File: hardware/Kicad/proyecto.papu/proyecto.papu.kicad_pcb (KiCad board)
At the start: 2 copper layers, 96.4 x 45.4 mm, 19 parts, among them J1 Conn_01x04, J2 Conn_01x03, J3 Screw_Terminal_01x02, J4 Screw_Terminal_01x02, J5 Screw_Terminal_01x02, SW1 SW_Nidec_CAS-120A1, SW2 SW_MEC_5E, U1 DRV8833_MODULE, U2 L7805

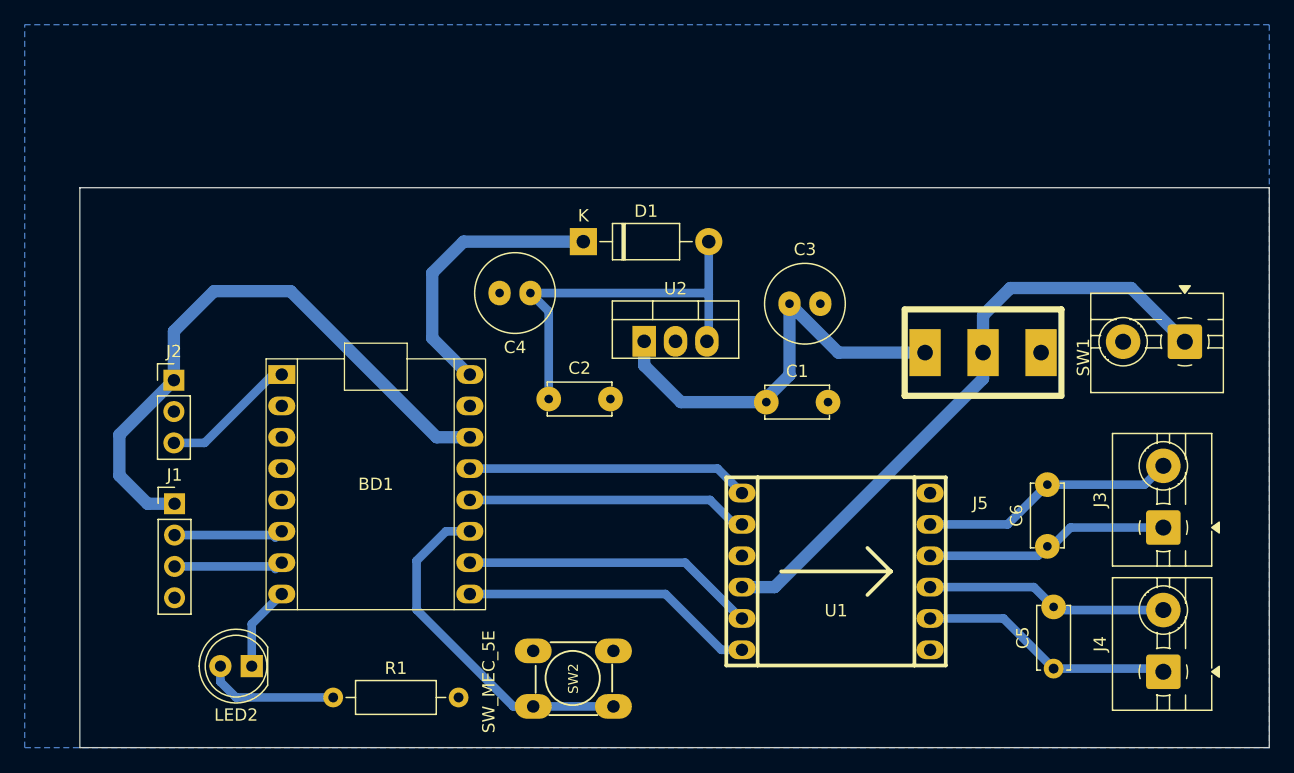
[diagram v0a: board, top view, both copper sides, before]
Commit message: se termino pcb
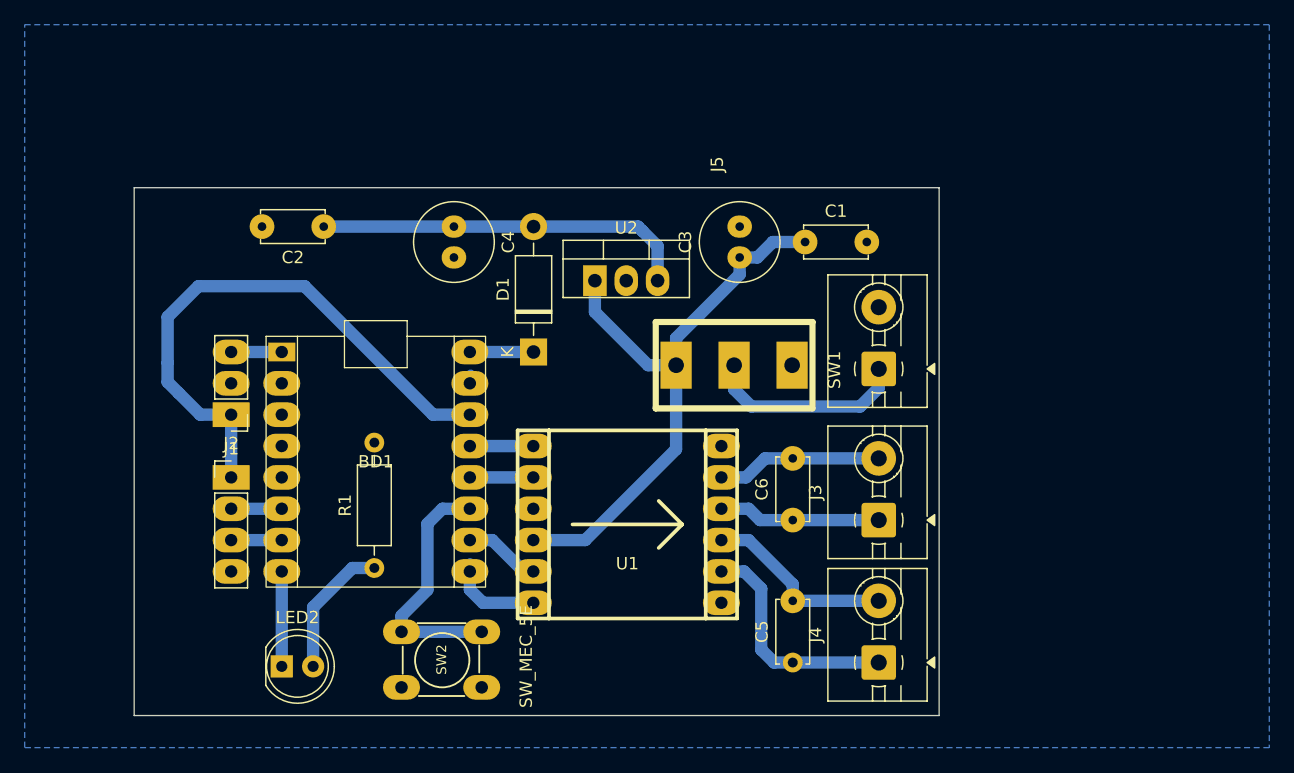
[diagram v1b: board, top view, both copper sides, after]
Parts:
- moved J5 24.9 mm to (150.0, 76.2), turned to 90 degrees
- moved J4 23.1 mm to (150.0, 100.0)
- moved J3 23.1 mm to (150.0, 88.5)
- moved C2 23.0 mm to (105.0, 64.7), turned to 180 degrees
- moved C5 21.1 mm to (143.0, 100.0)
- moved C6 20.7 mm to (143.0, 88.5)
- moved SW1 20.2 mm to (138.2, 76.0)
- moved U1 17.3 mm to (129.6, 88.8)
- moved C1 13.3 mm to (144.0, 66.0)
- moved R1 11.0 mm to (109.1, 92.4), turned to 90 degrees
- moved D1 9.81 mm to (122.0, 74.9), turned to 90 degrees
- moved C4 8.21 mm to (115.5, 64.7), turned to -90 degrees
- moved SW2 7.35 mm to (117.8, 97.5), turned to -90 degrees
- moved U2 6.33 mm to (129.7, 69.1)
- moved C3 5.51 mm to (138.7, 67.2), turned to 90 degrees
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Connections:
- J5 pad 1: 12v -> Net-(J5-Pin_1)
- SW1 pad 2: 12v -> Net-(J5-Pin_1)
- U1 pad 4: 12v -> +12V
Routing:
- net 12v: track 50.7 -> 0.00 mm
- net +5V: track 22.9 -> 5.16 mm
- net Motor 2 izq 1: track 23.9 -> 6.19 mm
- net Motor 1 Der1: track 22.9 -> 5.14 mm
- net Motor 1 Der 2: track 22.9 -> 5.14 mm
- net Motor 2 izq 2: track 23.9 -> 7.08 mm
- net Net-(J5-Pin_1): track 0.00 -> 16.4 mm
- net +12V: track 34.5 -> 49.0 mm
- net boton2: track 28.9 -> 20.1 mm
- net m11: track 20.9 -> 13.4 mm
- net trct5000: track 11.0 -> 4.10 mm
- net m10: track 19.8 -> 13.1 mm
- net trigg: track 9.63 -> 4.10 mm
- net echo: track 9.55 -> 4.10 mm
- net m9: track 20.0 -> 15.6 mm
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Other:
- board size 96.4 x 45.4 mm -> 65.2 x 42.8 mm
